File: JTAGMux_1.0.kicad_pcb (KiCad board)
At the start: 4 copper layers, 57.9 x 41.2 mm, 15 parts, among them J1 (Expension and configuration) Conn_02x10_Odd_Even, M1 MountingHole_3.7mm, M2 MountingHole_3.7mm, U1 SN74CBTLV16292DL

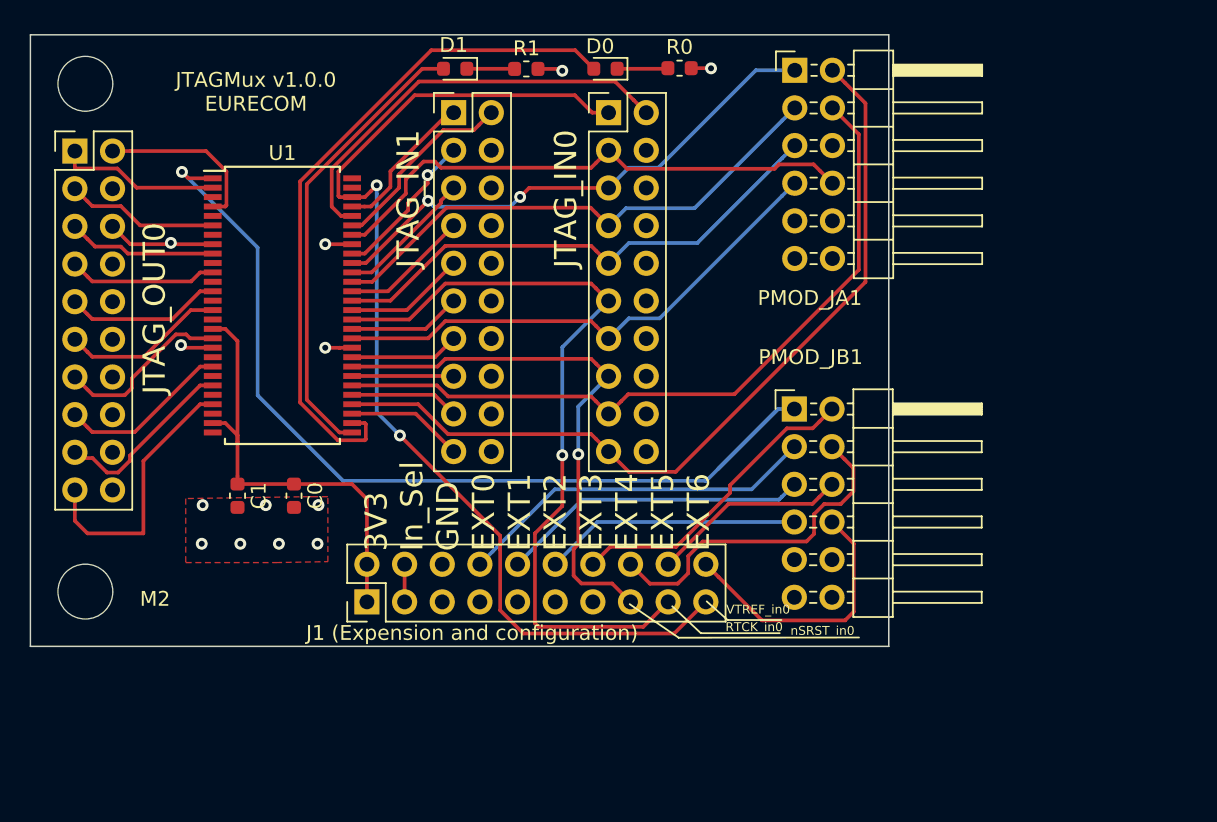
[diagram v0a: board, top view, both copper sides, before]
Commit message: version 1.0.1
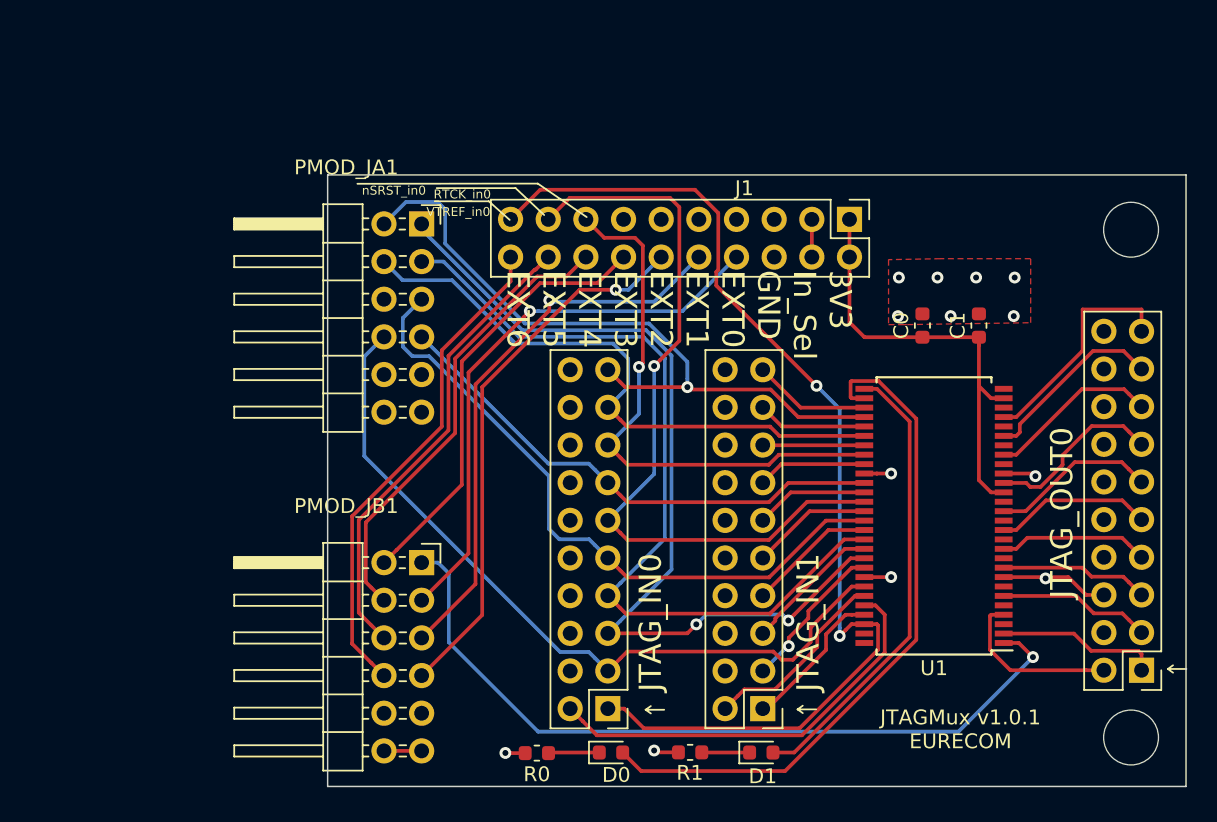
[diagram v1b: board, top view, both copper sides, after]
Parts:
- J1: renamed from J1 (Expension and configuration)
- moved M1 83.2 mm to (124.3, 156.0), turned to 180 degrees
- moved JTAG_OUT0 80.0 mm to (125.0, 151.5), turned to 180 degrees
- moved M2 74.6 mm to (124.3, 121.8), turned to 180 degrees
- moved C1 51.3 mm to (114.1, 128.3), turned to 90 degrees
- moved D1 50.5 mm to (99.4, 157.1), turned to 0 degrees
- moved R1 47.4 mm to (94.6, 157.1), turned to 180 degrees
- moved R0 47.2 mm to (84.3, 157.1), turned to 180 degrees
- moved U1 46.2 mm to (111.0, 141.1), turned to 180 degrees
- moved D0 46.1 mm to (89.3, 157.1), turned to 0 degrees
- moved JTAG_IN1 45.3 mm to (99.5, 154.1), turned to 180 degrees
- moved C0 43.9 mm to (110.3, 128.3), turned to 90 degrees
- moved J1 41.5 mm to (105.3, 121.1), turned to 270 degrees
- moved JTAG_IN0 40.2 mm to (89.0, 154.1), turned to 180 degrees
- moved PMOD_JA1 27.2 mm to (76.5, 121.4)
- moved PMOD_JB1 27.2 mm to (76.5, 144.2)
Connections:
- PMOD_JA1 pad 9: Net-(PMOD_JA1-Pad9) -> (no net)
- U1 pad 10: Net-(U1-Pad10) -> (no net)
- U1 pad 12: Net-(U1-Pad12) -> (no net)
- U1 pad 14: Net-(U1-Pad14) -> (no net)
- U1 pad 16: Net-(U1-Pad16) -> (no net)
- U1 pad 20: Net-(U1-Pad20) -> (no net)
- U1 pad 22: Net-(U1-Pad22) -> (no net)
- U1 pad 24: Net-(U1-Pad24) -> (no net)
- U1 pad 26: Net-(U1-Pad26) -> (no net)
- U1 pad 28: Net-(U1-Pad28) -> (no net)
- U1 pad 3: Net-(U1-Pad3) -> (no net)
- U1 pad 5: Net-(U1-Pad5) -> (no net)
- U1 pad 55: Net-(U1-Pad55) -> (no net)
- U1 pad 56: Net-(U1-Pad56) -> (no net)
- U1 pad 7: Net-(U1-Pad7) -> (no net)
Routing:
- net TDI_in0: track 35.6 -> 61.0 mm
- net TMS_in0: track 35.7 -> 56.6 mm
- net EXT2: track 17.3 -> 36.9 mm, vias 0 -> 1
- net EXT5: track 13.3 -> 31.7 mm
- net EXT1_IRQACK: track 20.9 -> 37.7 mm, vias 0 -> 1
- net EXT6: track 18.4 -> 33.5 mm
- net nTRST_in0: track 36.8 -> 51.7 mm
- net EXT0_IRQ: track 24.5 -> 38.0 mm, vias 0 -> 1
- net Select_input: track 65.8 -> 53.1 mm
- net DBACK_in0: track 57.0 -> 47.2 mm, vias 0 -> 1
- net TCK_in0: track 35.2 -> 45.0 mm
- net DBRQ_in0: track 50.7 -> 41.1 mm
- net EXT3: track 20.8 -> 29.6 mm
- net EXT4: track 23.2 -> 31.0 mm
- net DBACK_out: track 18.2 -> 15.4 mm
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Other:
- board text added: "JTAGMux v1.0.1 EURECOM"
- board text removed: "JTAGMux v1.0.0 EURECOM"
